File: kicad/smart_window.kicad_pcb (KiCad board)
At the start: 2 copper layers, 90 x 71.5 mm, 86 parts, among them J1 PROG, J10 LS2, J12 LS3, J13 Vmot1, J14 Vmot3, J2 Vmot2, J3 DOOR1, J4 MOT2, J5 MOT1, J6 MOT3, J7 I2C, J8 DOOR2, J9 LS1, Q10 BC807-40_215, Q11 BC817-40_215, Q12 BC807-40_215, Q13 BC817-40_215, Q15 BC817-40_215, Q17 BC807-40_215, Q18 BC817-40_215, Q19 BC807-40_215, Q20 BC817-40_215, Q22 BC817-40_215, Q24 BC807-40_215, Q25 BC817-40_215, Q26 BC807-40_215, Q27 BC817-40_215, Q4 BC817-40_215, U1 ESP-12F, U2 MP1584EN 3.3V, U3 LTV-817S, U4 LTV-817S, U5 LTV-817S, U6 LTV-817S, U7 LTV-817S, U8 LTV-817S

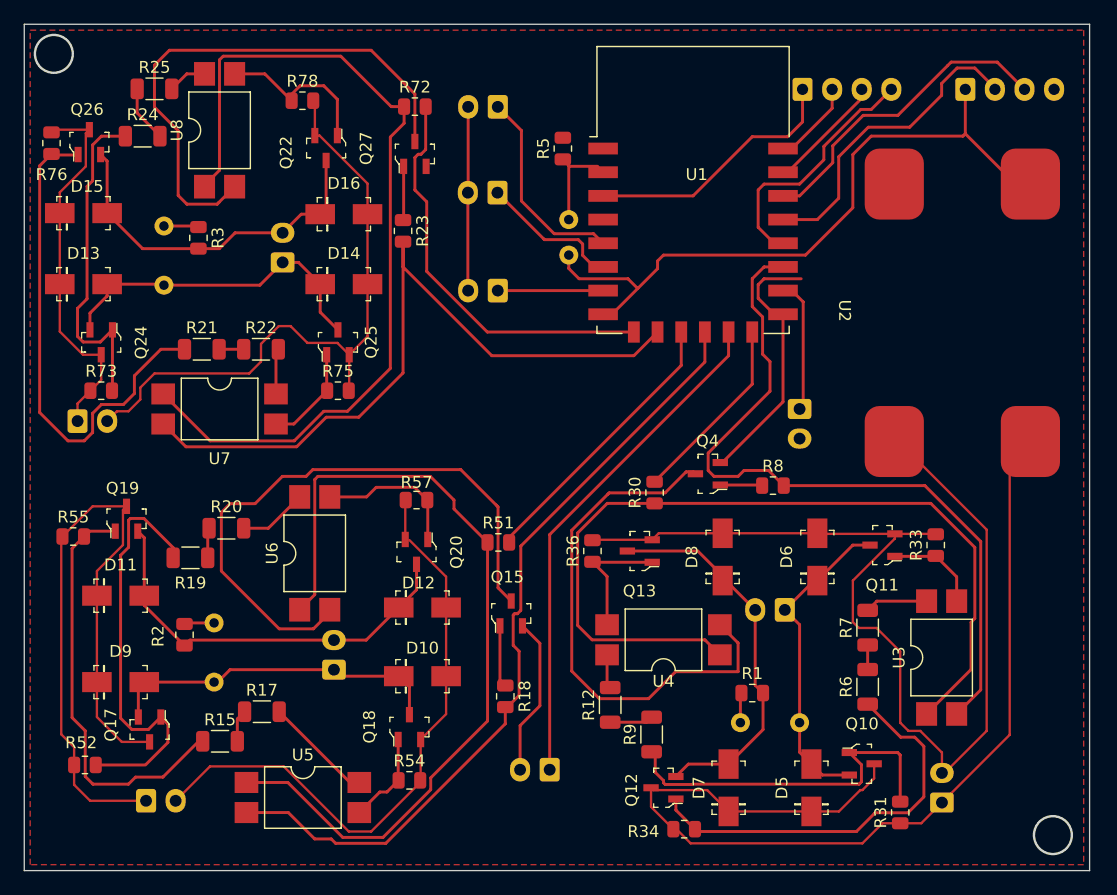
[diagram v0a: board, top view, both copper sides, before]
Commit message: вариант с микросхемами a4950
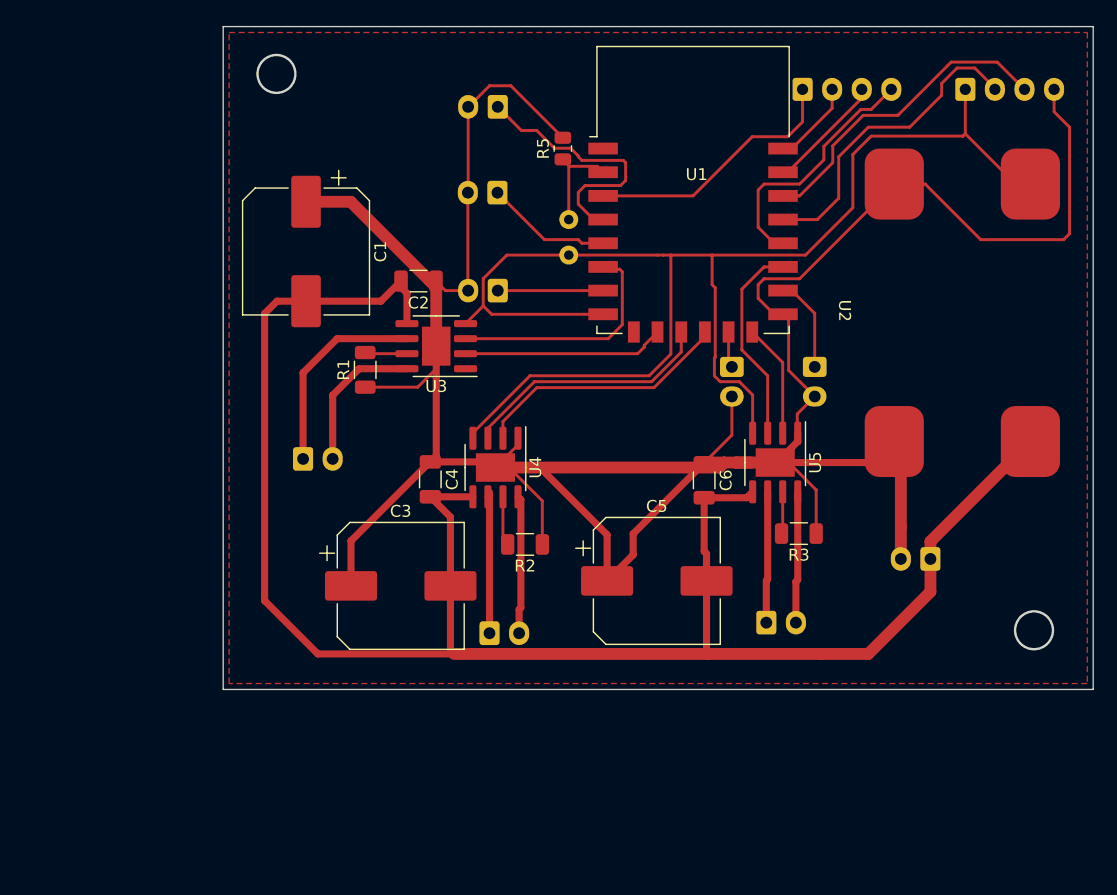
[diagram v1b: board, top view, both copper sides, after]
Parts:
- removed D10, D11, D12, D13, D14, D15, D16, D5, D6, D7, D8, D9: SS14, digikey-footprints:DO-214AC
- removed J14: Vmot3, Connector_JST:JST_XH_B2B-XH-A_1x02_P2.50mm_Vertical
- removed J2: Vmot2, Connector_JST:JST_XH_B2B-XH-A_1x02_P2.50mm_Vertical
- removed Q10, Q12, Q17, Q19, Q24, Q26: BC807-40_215, digikey-footprints:SOT-23-3
- removed Q11, Q13, Q15, Q18, Q20, Q22, Q25, Q27, Q4: BC817-40_215, digikey-footprints:SOT-23-3
- removed R12, R15, R17, R19, R20, R21, R22, R24, R25, R6, R7, R9: 1.2k, Resistor_SMD:R_1206_3216Metric
- removed R18, R23, R8: 1.5k, Resistor_SMD:R_0805_2012Metric
- removed R30, R51, R72: 100, Resistor_SMD:R_0805_2012Metric
- removed R31, R33, R34, R36, R52, R54, R55, R57, R73, R75, R76, R78: 1k, Resistor_SMD:R_0805_2012Metric
- removed U6, U7, U8: LTV-817S, Package_DIP:SMDIP-4_W9.53mm
- added C1: 100µF, Capacitor_SMD:CP_Elec_10x10.5, F.Cu at (36.0, 31.5)
- added C5: 100µF, Capacitor_SMD:CP_Elec_10x10.5, F.Cu at (65.6, 59.3)
- added C6: 0.22µF, Capacitor_SMD:C_1206_3216Metric, F.Cu at (69.6, 50.8)
- C2, C4: value C -> 0.22µF; footprint Capacitor_THT:C_Radial_D10.0mm_H16.0mm_P5.00mm -> Capacitor_SMD:C_1206_3216Metric; moved to F.Cu
- C3: value C -> 100µF; footprint Capacitor_THT:C_Radial_D10.0mm_H16.0mm_P5.00mm -> Capacitor_SMD:CP_Elec_10x10.5; moved to F.Cu
- R1, R2, R3: value 50 -> 0.2; footprint Resistor_SMD:R_0805_2012Metric -> Resistor_SMD:R_1206_3216Metric
- U3, U4, U5: value LTV-817S -> A4950E; footprint Package_DIP:SMDIP-4_W9.53mm -> Package_SO:SOIC-8-1EP_3.9x4.9mm_P1.27mm_EP2.41x3.3mm
- moved R3 56.5 mm to (77.6, 55.3), turned to 180 degrees
- moved J6 51.0 mm to (74.9, 62.9), turned to 0 degrees
- moved U3 50.1 mm to (47.0, 39.5), turned to 180 degrees
- moved C2 49.3 mm to (45.5, 34.0)
- moved U5 48.9 mm to (75.6, 49.3), turned to -90 degrees
- moved J5 42.6 mm to (35.8, 49.0), turned to 0 degrees
- moved R1 42.6 mm to (41.0, 41.5), turned to 90 degrees
- moved J10 37.3 mm to (72.0, 41.2), turned to -90 degrees
- moved R2 29.8 mm to (54.5, 56.2), turned to 180 degrees
- moved C4 27.8 mm to (46.5, 50.8), turned to -90 degrees
- moved J13 20.6 mm to (88.8, 57.5), turned to 180 degrees
- moved U4 20.3 mm to (52.0, 49.8), turned to -90 degrees
- moved C3 17.7 mm to (44.0, 59.8), turned to 0 degrees
- moved J4 13.5 mm to (51.5, 63.8), turned to 0 degrees
- moved J9 3.78 mm to (79.0, 41.2)
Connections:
- C2 pad 1: /h_bridge1/ML -> GND
- C2 pad 2: Net-(C2-Pad2) -> /24V+
- C3 pad 1: /h_bridge2/ML -> GND
- C3 pad 2: Net-(C3-Pad2) -> /24V+
- C4 pad 1: /h_bridge3/ML -> GND
- C4 pad 2: Net-(C4-Pad2) -> /24V+
- J13 pad 1: /24V+1 -> /24V+
- J13 pad 2: /24V-1 -> GND
- J4 pad 1: /h_bridge2/ML -> Net-(J4-Pad1)
- J4 pad 2: /h_bridge2/MR -> Net-(J4-Pad2)
- J5 pad 1: /h_bridge1/ML -> Net-(J5-Pad1)
- J5 pad 2: /h_bridge1/MR -> Net-(J5-Pad2)
- J6 pad 1: /h_bridge3/ML -> Net-(J6-Pad1)
- J6 pad 2: /h_bridge3/MR -> Net-(J6-Pad2)
- R1 pad 1: Net-(C2-Pad2) -> GND
- R1 pad 2: /h_bridge1/MR -> Net-(U3-Pad7)
- R2 pad 1: Net-(C3-Pad2) -> GND
- R2 pad 2: /h_bridge2/MR -> Net-(U4-Pad7)
- R3 pad 1: Net-(C4-Pad2) -> GND
- R3 pad 2: /h_bridge3/MR -> Net-(U5-Pad7)
- U1 pad 10: /M3_DIR -> /M1_DIR
- U1 pad 14: /M1_EN -> /M3_DIR
- U1 pad 17: /M1_DIR -> /M3_EN
- U1 pad 4: unconnected-(U1-Pad4) -> /DOOR1
- U1 pad 5: /DOOR1 -> /DOOR2
- U1 pad 6: /DOOR2 -> /M1_EN
- U1 pad 9: /M3_EN -> unconnected-(U1-Pad9)
- U2 pad 3: /24V+1 -> /24V+
- U2 pad 4: /24V-1 -> GND
- U3 pad 1: /h_bridge1/EN_IN -> GND
- U3 pad 3: Net-(Q11-Pad1) -> /M1_EN
- U3 pad 4: Net-(R7-Pad2) -> +3V3
- U4 pad 1: /h_bridge1/EN_IN -> GND
- U4 pad 2: /h_bridge1/CW_O -> /M2_DIR
- U4 pad 3: Net-(Q13-Pad1) -> /M2_EN
- U4 pad 4: Net-(R12-Pad2) -> +3V3
- U5 pad 1: /h_bridge2/EN_IN -> GND
- U5 pad 2: /M2_DIR -> /M3_DIR
- U5 pad 3: Net-(Q18-Pad1) -> /M3_EN
- U5 pad 4: Net-(R17-Pad2) -> +3V3
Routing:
- net GND: track 51.5 -> 260.8 mm
- net /24V+: track 0.00 -> 152.9 mm
- net /24V-1: track 88.7 -> 0.00 mm
- net /24V+1: track 84.3 -> 0.00 mm
- net /h_bridge3/EN_IN: track 74.7 -> 0.00 mm
- net /h_bridge1/EN_IN: track 72.7 -> 0.00 mm
- net /h_bridge2/EN_IN: track 71.0 -> 0.00 mm
- net +3V3: track 56.6 -> 118.8 mm
- net /24V+2: track 58.7 -> 0.00 mm
- net /24V-3: track 53.5 -> 0.00 mm
- net /M3_DIR: track 62.3 -> 9.62 mm
- net /24V-2: track 51.9 -> 0.00 mm
- net /h_bridge2/CW_O: track 51.5 -> 0.00 mm
- net /M1_DIR: track 63.3 -> 17.1 mm
- net /M2_DIR: track 67.9 -> 21.8 mm
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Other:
- board size 90 x 71.5 mm -> 73.5 x 56 mm
